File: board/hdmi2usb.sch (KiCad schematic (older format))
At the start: 0 parts

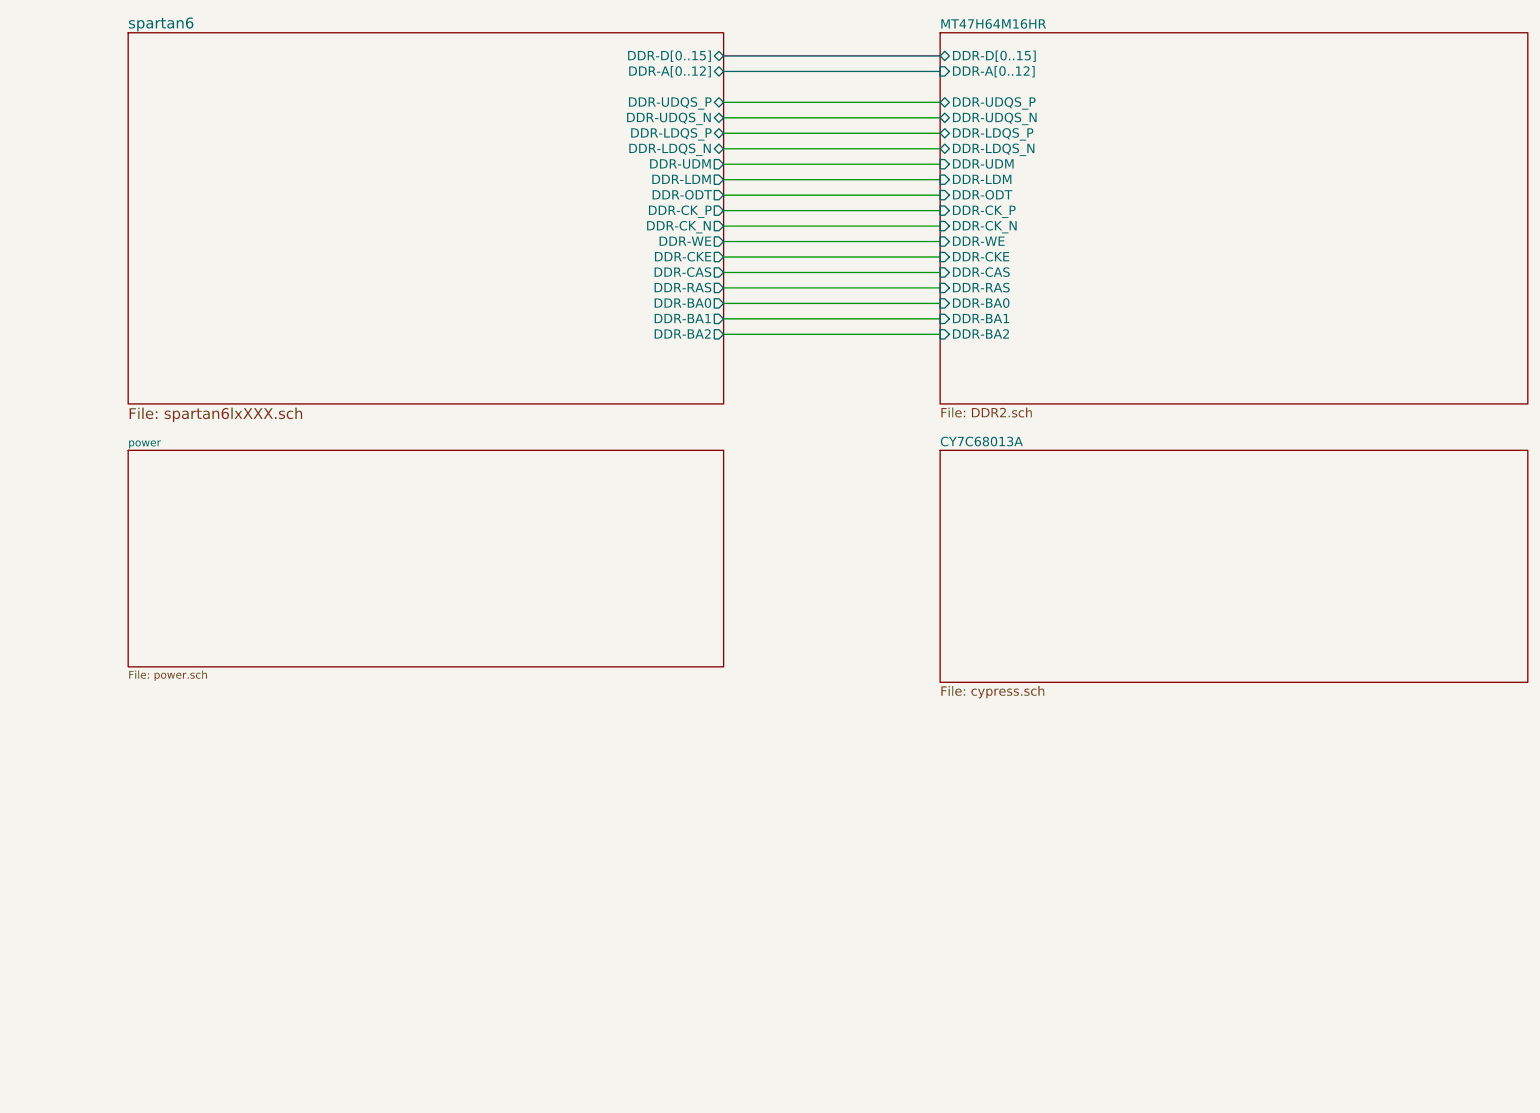
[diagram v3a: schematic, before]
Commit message: Issue #336
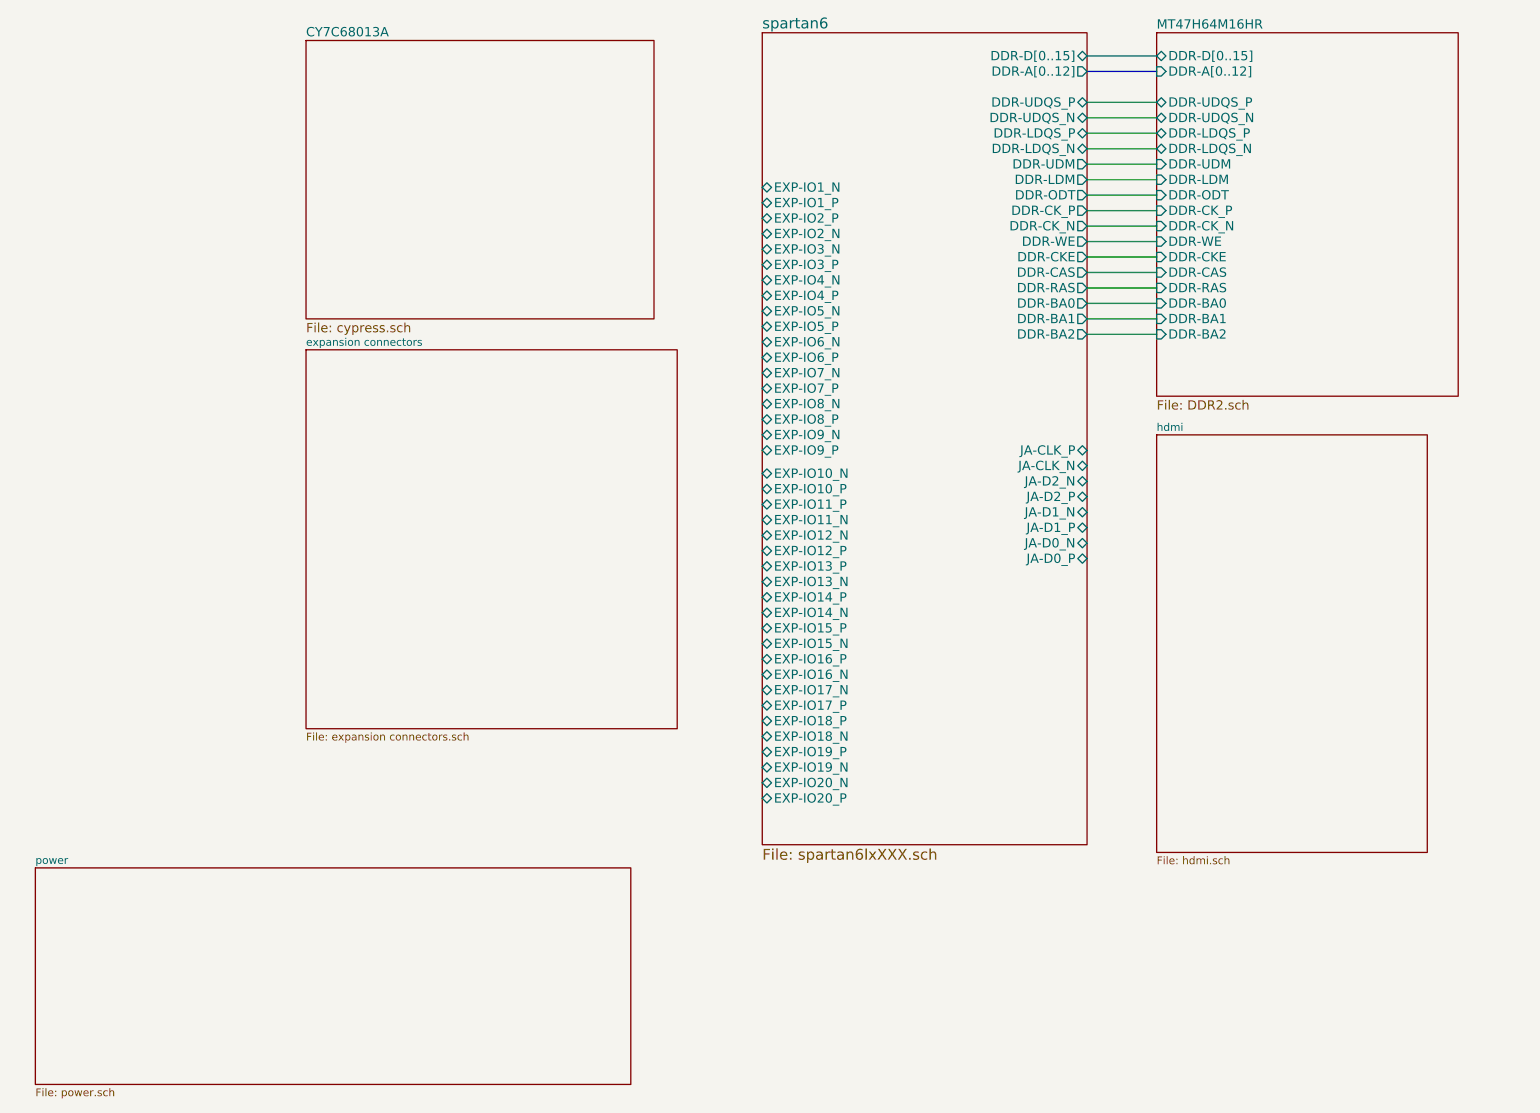
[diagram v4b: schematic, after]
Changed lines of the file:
@@
 LIBS:hdmi2usb
 LIBS:cypress-fx2
+LIBS:numato_kicad_lib
 LIBS:hdmi2usb-cache
 EELAYER 27 0
@@
 $Descr A4 11693 8268
 encoding utf-8
-Sheet 1 5
+Sheet 1 7
 Title ""
-Date "26 jun 2013"
+Date "27 jun 2013"
 Rev ""
 Comp ""
@@
 $EndDescr
 $Sheet
-S 7000 3400 3800 1500
+S 2900 750  2250 1800
 U 51B5BBC1
 F0 "CY7C68013A" 60
@@
 $EndSheet
 $Sheet
-S 1750 3400 3850 1400
+S 1150 6100 3850 1400
 U 51BACC6F
 F0 "power" 50
 F1 "power.sch" 50
 $EndSheet
-Wire Bus Line
-	7000 850  5600 850
-Wire Bus Line
-	7000 950  5600 950
+Wire Wire Line
+	7950 2650 8400 2650
+Wire Wire Line
+	7950 2550 8400 2550
+Wire Wire Line
+	7950 2450 8400 2450
+Wire Wire Line
+	7950 2350 8400 2350
+Wire Wire Line
+	7950 2250 8400 2250
+Wire Wire Line
+	7950 2150 8400 2150
+Wire Wire Line
+	7950 2050 8400 2050
+Wire Wire Line
+	7950 1950 8400 1950
+Wire Wire Line
+	7950 1850 8400 1850
+Wire Wire Line
+	7950 1750 8400 1750
+Wire Wire Line
+	7950 1650 8400 1650
+Wire Wire Line
+	7950 1550 8400 1550
+Wire Wire Line
+	7950 1450 8400 1450
+Wire Wire Line
+	7950 1350 8400 1350
+Wire Wire Line
+	7950 1250 8400 1250
 $Sheet
-S 7000 700  3800 2400
+S 8400 700  1950 2350
 U 51B846F4
 F0 "MT47H64M16HR" 60
 F1 "DDR2.sch" 60
-F2 "DDR-D[0..15]" B L 7000 850 60
-F3 "DDR-A[0..12]" I L 7000 950 60
-F4 "DDR-UDQS_P" B L 7000 1150 60
-F5 "DDR-UDQS_N" B L 7000 1250 60
-F6 "DDR-LDQS_P" B L 7000 1350 60
-F7 "DDR-LDQS_N" B L 7000 1450 60
-F8 "DDR-UDM" I L 7000 1550 60
-F9 "DDR-LDM" I L 7000 1650 60
-F10 "DDR-ODT" I L 7000 1750 60
-F11 "DDR-CK_P" I L 7000 1850 60
-F12 "DDR-CK_N" I L 7000 1950 60
-F13 "DDR-CKE" I L 7000 2150 60
-F14 "DDR-WE" I L 7000 2050 60
-F15 "DDR-CAS" I L 7000 2250 60
-F16 "DDR-RAS" I L 7000 2350 60
-F17 "DDR-BA0" I L 7000 2450 60
-F18 "DDR-BA1" I L 7000 2550 60
-F19 "DDR-BA2" I L 7000 2650 60
+F2 "DDR-D[0..15]" B L 8400 850 60
+F3 "DDR-A[0..12]" I L 8400 950 60
+F4 "DDR-UDQS_P" B L 8400 1150 60
+F5 "DDR-UDQS_N" B L 8400 1250 60
+F6 "DDR-LDQS_P" B L 8400 1350 60
+F7 "DDR-LDQS_N" B L 8400 1450 60
+F8 "DDR-UDM" I L 8400 1550 60
+F9 "DDR-LDM" I L 8400 1650 60
+F10 "DDR-ODT" I L 8400 1750 60
+F11 "DDR-CK_P" I L 8400 1850 60
+F12 "DDR-CK_N" I L 8400 1950 60
+F13 "DDR-CKE" I L 8400 2150 60
+F14 "DDR-WE" I L 8400 2050 60
+F15 "DDR-CAS" I L 8400 2250 60
+F16 "DDR-RAS" I L 8400 2350 60
+F17 "DDR-BA0" I L 8400 2450 60
+F18 "DDR-BA1" I L 8400 2550 60
+F19 "DDR-BA2" I L 8400 2650 60
+$EndSheet
+Wire Wire Line
+	7950 1150 8400 1150
+Wire Bus Line
+	7950 950  8400 950
+Wire Bus Line
+	7950 850  8400 850
+$Sheet
+S 8400 3300 1750 2700
+U 51CD5DED
+F0 "hdmi" 50
+F1 "hdmi.sch" 50
 $EndSheet
 $Sheet
-S 1750 700  3850 2400
+S 2900 2750 2400 2450
+U 51CD6077
+F0 "expansion connectors" 50
+F1 "expansion connectors.sch" 50
+$EndSheet
+$Sheet
+S 5850 700  2100 5250
 U 51AED6DE
 F0 "spartan6" 70
 F1 "spartan6lxXXX.sch" 70
-F2 "DDR-D[0..15]" B R 5600 850 60
-F3 "DDR-A[0..12]" B R 5600 950 60
-F4 "DDR-LDQS_P" B R 5600 1350 60
-F5 "DDR-LDQS_N" B R 5600 1450 60
-F6 "DDR-UDM" O R 5600 1550 60
-F7 "DDR-LDM" O R 5600 1650 60
-F8 "DDR-UDQS_P" B R 5600 1150 60
-F9 "DDR-UDQS_N" B R 5600 1250 60
-F10 "DDR-RAS" O R 5600 2350 60
-F11 "DDR-CAS" O R 5600 2250 60
-F12 "DDR-ODT" O R 5600 1750 60
-F13 "DDR-CK_P" O R 5600 1850 60
-F14 "DDR-CK_N" O R 5600 1950 60
-F15 "DDR-BA0" O R 5600 2450 60
-F16 "DDR-BA1" O R 5600 2550 60
-F17 "DDR-WE" O R 5600 2050 60
-F18 "DDR-BA2" O R 5600 2650 60
-F19 "DDR-CKE" O R 5600 2150 60
+F2 "DDR-D[0..15]" B R 7950 850 60
+F3 "DDR-A[0..12]" O R 7950 950 60
+F4 "DDR-LDQS_P" B R 7950 1350 60
+F5 "DDR-LDQS_N" B R 7950 1450 60
+F6 "DDR-UDM" O R 7950 1550 60
+F7 "DDR-LDM" O R 7950 1650 60
+F8 "DDR-UDQS_P" B R 7950 1150 60
+F9 "DDR-UDQS_N" B R 7950 1250 60
+F10 "DDR-RAS" O R 7950 2350 60
+F11 "DDR-CAS" O R 7950 2250 60
+F12 "DDR-ODT" O R 7950 1750 60
+F13 "DDR-CK_P" O R 7950 1850 60
+F14 "DDR-CK_N" O R 7950 1950 60
+F15 "DDR-BA0" O R 7950 2450 60
+F16 "DDR-BA1" O R 7950 2550 60
+F17 "DDR-WE" O R 7950 2050 60
+F18 "DDR-BA2" O R 7950 2650 60
+F19 "DDR-CKE" O R 7950 2150 60
+F20 "EXP-IO1_N" B L 5850 1700 60
+F21 "EXP-IO1_P" B L 5850 1800 60
+F22 "EXP-IO10_N" B L 5850 3550 60
+F23 "EXP-IO10_P" B L 5850 3650 60
+F24 "EXP-IO11_P" B L 5850 3750 60
+F25 "EXP-IO11_N" B L 5850 3850 60
+F26 "EXP-IO12_N" B L 5850 3950 60
+F27 "EXP-IO12_P" B L 5850 4050 60
+F28 "JA-CLK_P" B R 7950 3400 60
+F29 "JA-CLK_N" B R 7950 3500 60
+F30 "EXP-IO13_P" B L 5850 4150 60
+F31 "EXP-IO13_N" B L 5850 4250 60
+F32 "EXP-IO14_P" B L 5850 4350 60
+F33 "EXP-IO14_N" B L 5850 4450 60
+F34 "JA-D2_N" B R 7950 3600 60
+F35 "JA-D2_P" B R 7950 3700 60
+F36 "JA-D1_N" B R 7950 3800 60
+F37 "JA-D1_P" B R 7950 3900 60
+F38 "JA-D0_N" B R 7950 4000 60
+F39 "JA-D0_P" B R 7950 4100 60
+F40 "EXP-IO15_P" B L 5850 4550 60
+F41 "EXP-IO15_N" B L 5850 4650 60
+F42 "EXP-IO16_P" B L 5850 4750 60
+F43 "EXP-IO16_N" B L 5850 4850 60
+F44 "EXP-IO17_N" B L 5850 4950 60
+F45 "EXP-IO17_P" B L 5850 5050 60
+F46 "EXP-IO18_P" B L 5850 5150 60
+F47 "EXP-IO18_N" B L 5850 5250 60
+F48 "EXP-IO19_P" B L 5850 5350 60
+F49 "EXP-IO19_N" B L 5850 5450 60
+F50 "EXP-IO2_P" B L 5850 1900 60
+F51 "EXP-IO2_N" B L 5850 2000 60
+F52 "EXP-IO20_N" B L 5850 5550 60
+F53 "EXP-IO20_P" B L 5850 5650 60
+F54 "EXP-IO3_N" B L 5850 2100 60
+F55 "EXP-IO3_P" B L 5850 2200 60
+F56 "EXP-IO4_N" B L 5850 2300 60
+F57 "EXP-IO4_P" B L 5850 2400 60
+F58 "EXP-IO5_N" B L 5850 2500 60
+F59 "EXP-IO5_P" B L 5850 2600 60
+F60 "EXP-IO6_N" B L 5850 2700 60
+F61 "EXP-IO6_P" B L 5850 2800 60
+F62 "EXP-IO7_N" B L 5850 2900 60
+F63 "EXP-IO7_P" B L 5850 3000 60
+F64 "EXP-IO8_N" B L 5850 3100 60
+F65 "EXP-IO8_P" B L 5850 3200 60
+F66 "EXP-IO9_N" B L 5850 3300 60
+F67 "EXP-IO9_P" B L 5850 3400 60
 $EndSheet
-Wire Wire Line
-	5600 1150 7000 1150
-Wire Wire Line
-	7000 1250 5600 1250
-Wire Wire Line
-	5600 1350 7000 1350
-Wire Wire Line
-	7000 1450 5600 1450
-Wire Wire Line
-	5600 1550 7000 1550
-Wire Wire Line
-	7000 1650 5600 1650
-Wire Wire Line
-	5600 1750 7000 1750
-Wire Wire Line
-	7000 1850 5600 1850
-Wire Wire Line
-	5600 1950 7000 1950
-Wire Wire Line
-	5600 2050 7000 2050
-Wire Wire Line
-	5600 2150 7000 2150
-Wire Wire Line
-	7000 2250 5600 2250
-Wire Wire Line
-	5600 2350 7000 2350
-Wire Wire Line
-	5600 2450 7000 2450
-Wire Wire Line
-	7000 2550 5600 2550
-Wire Wire Line
-	5600 2650 7000 2650
 $EndSCHEMATC

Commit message: Issue #336
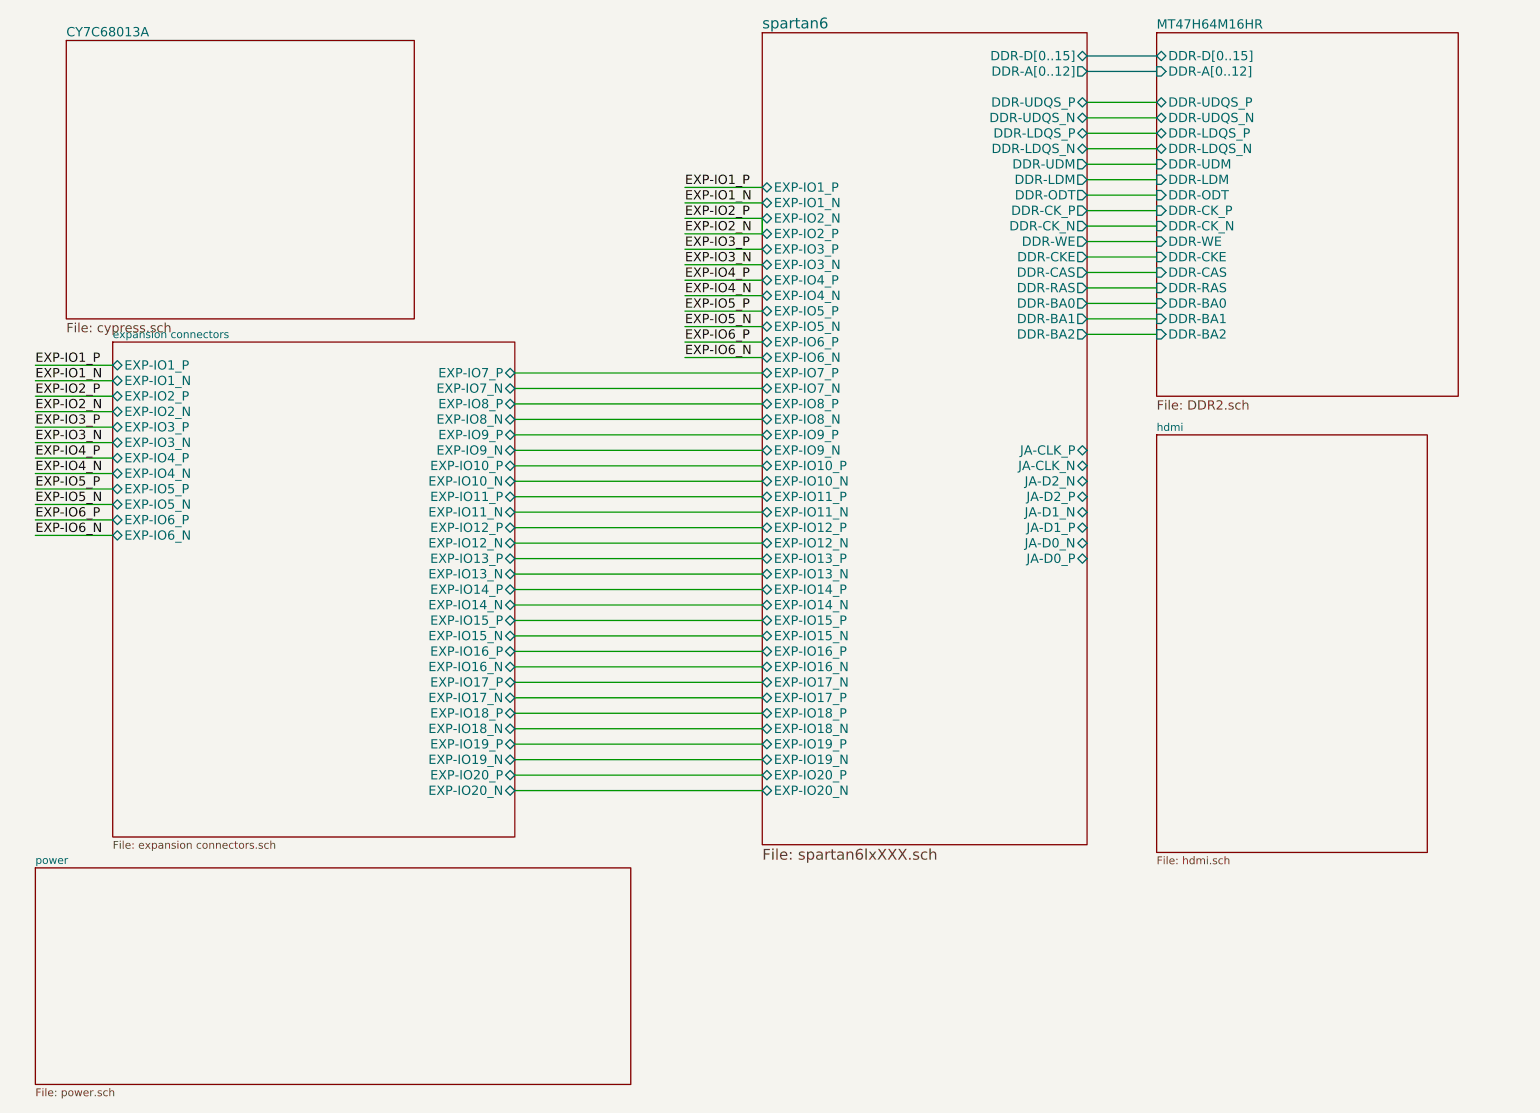
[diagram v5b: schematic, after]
